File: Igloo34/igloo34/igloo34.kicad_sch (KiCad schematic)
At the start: 24 parts, among them J1 BE40A-S-92SP-2-2-08-0152, J10 Conn_01x10, J11 LSHM-120-02.5-L-DV-A-S-TR, J12 LSHM-120-02.5-L-DV-A-S-TR, J13 Conn_01x10, J14 Conn_01x10, J16 Conn_01x02, J17 Conn_01x02, J18 Conn_01x02, J19 Conn_01x02, J2 Conn_01x08_Pin, J21 Conn_01x02, J22 Conn_01x02, J23 Conn_01x02, J24 Conn_01x02, J3 BE40A-S-92SP-2-2-08-0152, J4 Conn_01x08_Pin, J5 Conn_01x08_Pin, J6 Conn_01x08_Pin, J7 LSHM-120-02.5-L-DV-A-S-TR, J8 Conn_01x10, J9 LSHM-120-02.5-L-DV-A-S-TR

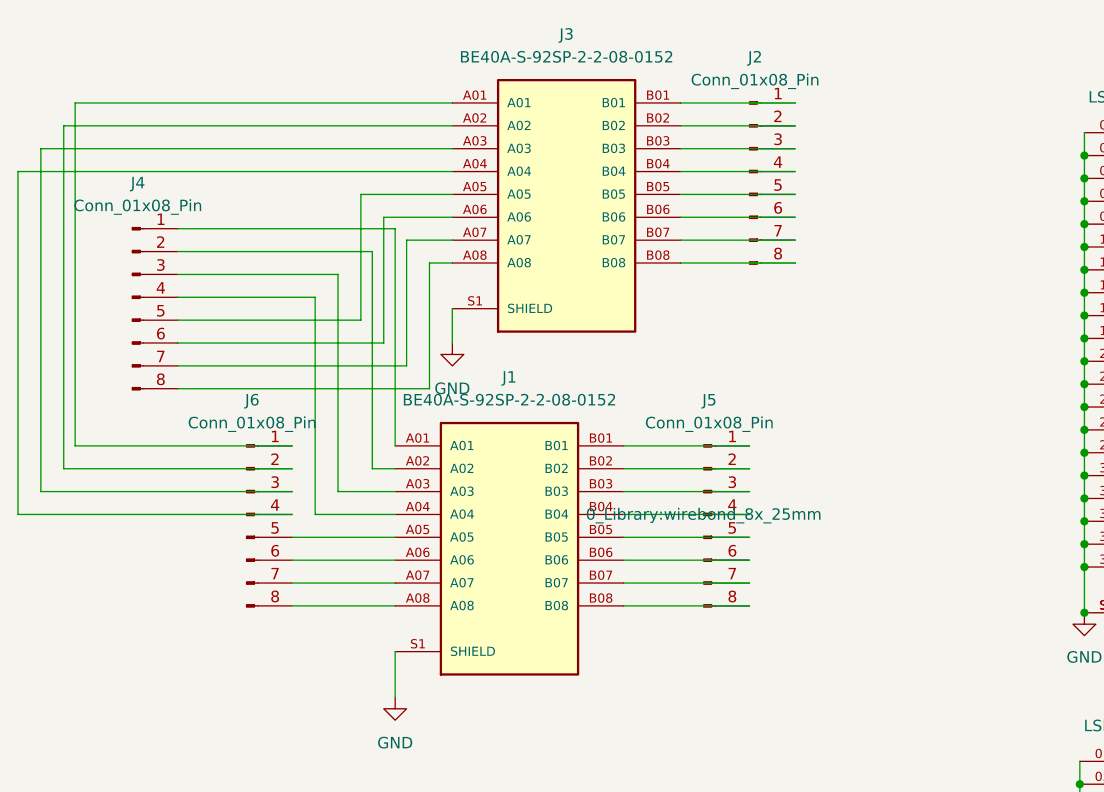
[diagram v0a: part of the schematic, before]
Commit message: update
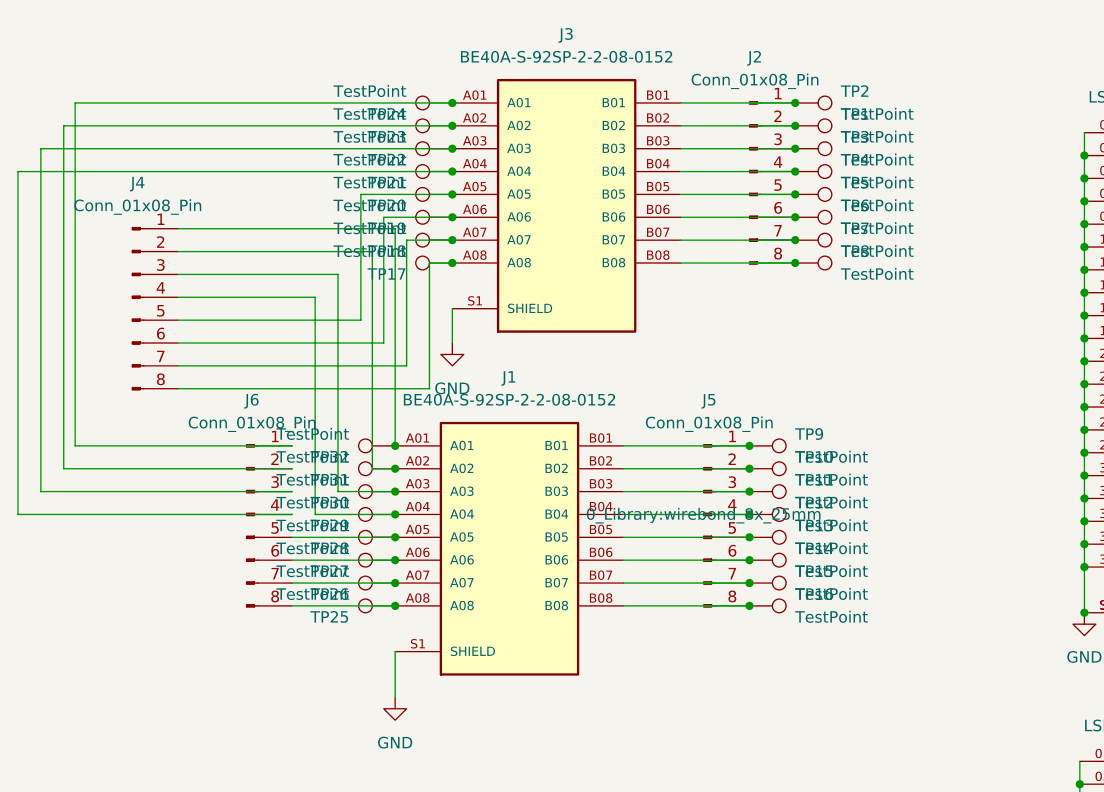
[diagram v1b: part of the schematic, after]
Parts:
- added TP1, TP10, TP11, TP12, TP13, TP14, TP15, TP16, TP17, TP18, TP19, TP2, TP20, TP21, TP22, TP23, TP24, TP25, TP26, TP27, TP28, TP29, TP3, TP30, TP31, TP32, TP4, TP5, TP6, TP7, TP8, TP9: TestPoint, TestPoint:TestPoint_THTPad_D1.0mm_Drill0.5mm, symbol Connector:TestPoint
- J11, J12, J7, J9: LCSC (none) -> C3654193
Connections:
- net at J1.B01, J5.1 (Pin_1): now also TP9.1
- net at J1.B02, J5.2 (Pin_2): now also TP10.1
- net at J1.B03, J5.3 (Pin_3): now also TP11.1
- net at J1.B04, J5.4 (Pin_4): now also TP12.1
- net at J1.B05, J5.5 (Pin_5): now also TP13.1
- net at J1.B06, J5.6 (Pin_6): now also TP14.1
- net at J1.B07, J5.7 (Pin_7): now also TP15.1
- net at J1.B08, J5.8 (Pin_8): now also TP16.1
- net at J2.1 (Pin_1), J3.B01: now also TP2.1
- net at J2.2 (Pin_2), J3.B02: now also TP1.1
- net at J2.3 (Pin_3), J3.B03: now also TP3.1
- net at J2.4 (Pin_4), J3.B04: now also TP4.1
- net at J2.5 (Pin_5), J3.B05: now also TP5.1
- net at J2.6 (Pin_6), J3.B06: now also TP6.1
- net at J2.7 (Pin_7), J3.B07: now also TP7.1
- net at J2.8 (Pin_8), J3.B08: now also TP8.1
- net at J3.A01, J6.1 (Pin_1): now also TP24.1
- net at J3.A02, J6.2 (Pin_2): now also TP23.1
- net at J3.A03, J6.3 (Pin_3): now also TP22.1
- net at J3.A04, J6.4 (Pin_4): now also TP21.1
- net at J1.A05, J6.5 (Pin_5): now also TP28.1
- net at J1.A06, J6.6 (Pin_6): now also TP27.1
- net at J1.A07, J6.7 (Pin_7): now also TP26.1
- net at J1.A08, J6.8 (Pin_8): now also TP25.1
- net at J1.A01, J4.1 (Pin_1): now also TP32.1
- net at J1.A02, J4.2 (Pin_2): now also TP31.1
- net at J1.A03, J4.3 (Pin_3): now also TP30.1
- net at J1.A04, J4.4 (Pin_4): now also TP29.1
- net at J3.A05, J4.5 (Pin_5): now also TP20.1
- net at J3.A06, J4.6 (Pin_6): now also TP19.1
- net at J3.A07, J4.7 (Pin_7): now also TP18.1
- net at J3.A08, J4.8 (Pin_8): now also TP17.1

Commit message: update
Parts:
- TP1, TP10, TP11, TP12, TP13, TP14, TP15, TP16, TP17, TP18, TP19, TP2, TP20, TP21, TP22, TP23, TP24, TP25, TP26, TP27, TP28, TP29, TP3, TP30, TP31, TP32, TP4, TP5, TP6, TP7, TP8, TP9: footprint TestPoint:TestPoint_THTPad_D1.0mm_Drill0.5mm -> 0_Library:Test point top pad
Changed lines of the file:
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@@
       (effects (font (size 1.27 1.27)) (justify left))
     )
-    (property "Footprint" "TestPoint:TestPoint_THTPad_D1.0mm_Drill0.5mm" (at 59.69 76.2 0)
+    (property "Footprint" "0_Library:Test point top pad" (at 59.69 76.2 0)
       (effects (font (size 1.27 1.27)) hide)
     )
@@
       (effects (font (size 1.27 1.27)) (justify left))
     )
-    (property "Footprint" "TestPoint:TestPoint_THTPad_D1.0mm_Drill0.5mm" (at 99.06 88.9 0)
+    (property "Footprint" "0_Library:Test point top pad" (at 99.06 88.9 0)
       (effects (font (size 1.27 1.27)) hide)
     )
@@
       (effects (font (size 1.27 1.27)) (justify left))
     )
-    (property "Footprint" "TestPoint:TestPoint_THTPad_D1.0mm_Drill0.5mm" (at 59.69 68.58 0)
+    (property "Footprint" "0_Library:Test point top pad" (at 59.69 68.58 0)
       (effects (font (size 1.27 1.27)) hide)
     )
@@
       (effects (font (size 1.27 1.27)) (justify left))
     )
-    (property "Footprint" "TestPoint:TestPoint_THTPad_D1.0mm_Drill0.5mm" (at 104.14 50.8 0)
+    (property "Footprint" "0_Library:Test point top pad" (at 104.14 50.8 0)
       (effects (font (size 1.27 1.27)) hide)
     )
@@
       (effects (font (size 1.27 1.27)) (justify left))
     )
-    (property "Footprint" "TestPoint:TestPoint_THTPad_D1.0mm_Drill0.5mm" (at 99.06 73.66 0)
+    (property "Footprint" "0_Library:Test point top pad" (at 99.06 73.66 0)
       (effects (font (size 1.27 1.27)) hide)
     )
@@
       (effects (font (size 1.27 1.27)) (justify left))
     )
-    (property "Footprint" "TestPoint:TestPoint_THTPad_D1.0mm_Drill0.5mm" (at 66.04 38.1 0)
+    (property "Footprint" "0_Library:Test point top pad" (at 66.04 38.1 0)
       (effects (font (size 1.27 1.27)) hide)
     )
@@
       (effects (font (size 1.27 1.27)) (justify left))
     )
-    (property "Footprint" "TestPoint:TestPoint_THTPad_D1.0mm_Drill0.5mm" (at 66.04 33.02 0)
+    (property "Footprint" "0_Library:Test point top pad" (at 66.04 33.02 0)
       (effects (font (size 1.27 1.27)) hide)
     )
@@
       (effects (font (size 1.27 1.27)) (justify left))
     )
-    (property "Footprint" "TestPoint:TestPoint_THTPad_D1.0mm_Drill0.5mm" (at 66.04 35.56 0)
+    (property "Footprint" "0_Library:Test point top pad" (at 66.04 35.56 0)
       (effects (font (size 1.27 1.27)) hide)
     )
@@
       (effects (font (size 1.27 1.27)) (justify left))
     )
-    (property "Footprint" "TestPoint:TestPoint_THTPad_D1.0mm_Drill0.5mm" (at 59.69 60.96 0)
+    (property "Footprint" "0_Library:Test point top pad" (at 59.69 60.96 0)
       (effects (font (size 1.27 1.27)) hide)
     )
@@
       (effects (font (size 1.27 1.27)) (justify left))
     )
-    (property "Footprint" "TestPoint:TestPoint_THTPad_D1.0mm_Drill0.5mm" (at 99.06 78.74 0)
+    (property "Footprint" "0_Library:Test point top pad" (at 99.06 78.74 0)
       (effects (font (size 1.27 1.27)) hide)
     )
@@
       (effects (font (size 1.27 1.27)) (justify left))
     )
-    (property "Footprint" "TestPoint:TestPoint_THTPad_D1.0mm_Drill0.5mm" (at 104.14 38.1 0)
+    (property "Footprint" "0_Library:Test point top pad" (at 104.14 38.1 0)
       (effects (font (size 1.27 1.27)) hide)
     )
@@
       (effects (font (size 1.27 1.27)) (justify left))
     )
-    (property "Footprint" "TestPoint:TestPoint_THTPad_D1.0mm_Drill0.5mm" (at 59.69 66.04 0)
+    (property "Footprint" "0_Library:Test point top pad" (at 59.69 66.04 0)
       (effects (font (size 1.27 1.27)) hide)
     )
@@
       (effects (font (size 1.27 1.27)) (justify left))
     )
-    (property "Footprint" "TestPoint:TestPoint_THTPad_D1.0mm_Drill0.5mm" (at 104.14 33.02 0)
+    (property "Footprint" "0_Library:Test point top pad" (at 104.14 33.02 0)
       (effects (font (size 1.27 1.27)) hide)
     )
@@
       (effects (font (size 1.27 1.27)) (justify left))
     )
-    (property "Footprint" "TestPoint:TestPoint_THTPad_D1.0mm_Drill0.5mm" (at 104.14 35.56 0)
+    (property "Footprint" "0_Library:Test point top pad" (at 104.14 35.56 0)
       (effects (font (size 1.27 1.27)) hide)
     )
@@
       (effects (font (size 1.27 1.27)) (justify left))
     )
-    (property "Footprint" "TestPoint:TestPoint_THTPad_D1.0mm_Drill0.5mm" (at 104.14 40.64 0)
+    (property "Footprint" "0_Library:Test point top pad" (at 104.14 40.64 0)
       (effects (font (size 1.27 1.27)) hide)
     )
@@
       (effects (font (size 1.27 1.27)) (justify left))
     )
-    (property "Footprint" "TestPoint:TestPoint_THTPad_D1.0mm_Drill0.5mm" (at 59.69 78.74 0)
+    (property "Footprint" "0_Library:Test point top pad" (at 59.69 78.74 0)
       (effects (font (size 1.27 1.27)) hide)
     )
@@
       (effects (font (size 1.27 1.27)) (justify left))
     )
-    (property "Footprint" "TestPoint:TestPoint_THTPad_D1.0mm_Drill0.5mm" (at 59.69 73.66 0)
+    (property "Footprint" "0_Library:Test point top pad" (at 59.69 73.66 0)
       (effects (font (size 1.27 1.27)) hide)
     )
@@
       (effects (font (size 1.27 1.27)) (justify left))
     )
-    (property "Footprint" "TestPoint:TestPoint_THTPad_D1.0mm_Drill0.5mm" (at 104.14 45.72 0)
+    (property "Footprint" "0_Library:Test point top pad" (at 104.14 45.72 0)
       (effects (font (size 1.27 1.27)) hide)
     )
@@
       (effects (font (size 1.27 1.27)) (justify left))
     )
-    (property "Footprint" "TestPoint:TestPoint_THTPad_D1.0mm_Drill0.5mm" (at 99.06 76.2 0)
+    (property "Footprint" "0_Library:Test point top pad" (at 99.06 76.2 0)
       (effects (font (size 1.27 1.27)) hide)
     )
@@
       (effects (font (size 1.27 1.27)) (justify left))
     )
-    (property "Footprint" "TestPoint:TestPoint_THTPad_D1.0mm_Drill0.5mm" (at 104.14 43.18 0)
+    (property "Footprint" "0_Library:Test point top pad" (at 104.14 43.18 0)
       (effects (font (size 1.27 1.27)) hide)
     )
@@
       (effects (font (size 1.27 1.27)) (justify left))
     )
-    (property "Footprint" "TestPoint:TestPoint_THTPad_D1.0mm_Drill0.5mm" (at 66.04 25.4 0)
+    (property "Footprint" "0_Library:Test point top pad" (at 66.04 25.4 0)
       (effects (font (size 1.27 1.27)) hide)
     )
@@
       (effects (font (size 1.27 1.27)) (justify left))
     )
-    (property "Footprint" "TestPoint:TestPoint_THTPad_D1.0mm_Drill0.5mm" (at 66.04 27.94 0)
+    (property "Footprint" "0_Library:Test point top pad" (at 66.04 27.94 0)
       (effects (font (size 1.27 1.27)) hide)
     )
@@
       (effects (font (size 1.27 1.27)) (justify left))
     )
-    (property "Footprint" "TestPoint:TestPoint_THTPad_D1.0mm_Drill0.5mm" (at 59.69 63.5 0)
+    (property "Footprint" "0_Library:Test point top pad" (at 59.69 63.5 0)
       (effects (font (size 1.27 1.27)) hide)
     )
@@
       (effects (font (size 1.27 1.27)) (justify left))
     )
-    (property "Footprint" "TestPoint:TestPoint_THTPad_D1.0mm_Drill0.5mm" (at 99.06 86.36 0)
+    (property "Footprint" "0_Library:Test point top pad" (at 99.06 86.36 0)
       (effects (font (size 1.27 1.27)) hide)
     )
@@
       (effects (font (size 1.27 1.27)) (justify left))
     )
-    (property "Footprint" "TestPoint:TestPoint_THTPad_D1.0mm_Drill0.5mm" (at 99.06 81.28 0)
+    (property "Footprint" "0_Library:Test point top pad" (at 99.06 81.28 0)
       (effects (font (size 1.27 1.27)) hide)
     )
@@
       (effects (font (size 1.27 1.27)) (justify left))
     )
-    (property "Footprint" "TestPoint:TestPoint_THTPad_D1.0mm_Drill0.5mm" (at 66.04 40.64 0)
+    (property "Footprint" "0_Library:Test point top pad" (at 66.04 40.64 0)
       (effects (font (size 1.27 1.27)) hide)
     )
@@
       (effects (font (size 1.27 1.27)) (justify left))
     )
-    (property "Footprint" "TestPoint:TestPoint_THTPad_D1.0mm_Drill0.5mm" (at 59.69 71.12 0)
+    (property "Footprint" "0_Library:Test point top pad" (at 59.69 71.12 0)
       (effects (font (size 1.27 1.27)) hide)
     )
@@
       (effects (font (size 1.27 1.27)) (justify left))
     )
-    (property "Footprint" "TestPoint:TestPoint_THTPad_D1.0mm_Drill0.5mm" (at 66.04 22.86 0)
+    (property "Footprint" "0_Library:Test point top pad" (at 66.04 22.86 0)
       (effects (font (size 1.27 1.27)) hide)
     )
@@
       (effects (font (size 1.27 1.27)) (justify left))
     )
-    (property "Footprint" "TestPoint:TestPoint_THTPad_D1.0mm_Drill0.5mm" (at 66.04 30.48 0)
+    (property "Footprint" "0_Library:Test point top pad" (at 66.04 30.48 0)
       (effects (font (size 1.27 1.27)) hide)
     )
@@
       (effects (font (size 1.27 1.27)) (justify left))
     )
-    (property "Footprint" "TestPoint:TestPoint_THTPad_D1.0mm_Drill0.5mm" (at 104.14 48.26 0)
+    (property "Footprint" "0_Library:Test point top pad" (at 104.14 48.26 0)
       (effects (font (size 1.27 1.27)) hide)
     )
@@
       (effects (font (size 1.27 1.27)) (justify left))
     )
-    (property "Footprint" "TestPoint:TestPoint_THTPad_D1.0mm_Drill0.5mm" (at 99.06 71.12 0)
+    (property "Footprint" "0_Library:Test point top pad" (at 99.06 71.12 0)
       (effects (font (size 1.27 1.27)) hide)
     )
@@
       (effects (font (size 1.27 1.27)) (justify left))
     )
-    (property "Footprint" "TestPoint:TestPoint_THTPad_D1.0mm_Drill0.5mm" (at 99.06 83.82 0)
-      (effects (font (size 1.27 1.27)) hide)
-    )
+    (property "Footprint" "0_Library:Test point top pad" (at 99.06 83.82 0)
+      (effects (font (size 1.27 1.27)) hide)
+    )

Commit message: increased via sizes
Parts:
- J9: LCSC (none) -> C3654193
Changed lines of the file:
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@@
       (effects (font (size 1.27 1.27)) (justify bottom) hide)
+    )
+    (property "LCSC" "C3654193" (at 39.37 209.55 0)
+      (effects (font (size 1.27 1.27)) hide)
     )
     (pin "01")
